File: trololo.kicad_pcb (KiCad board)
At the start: 4 copper layers, 136 x 54.8 mm, 101 parts, among them J1 USB_OTG, J10 Conn_02x12_Odd_Even, J11 Conn_02x02_Odd_Even, J13 PROTO1, J18 PROTO1, J2 USB_OTG, J3 Wuerth_7499010121A, J4 Micro_SD_Card, J5 Screw_Terminal_01x06, J6 Conn_02x12_Odd_Even, J7 USB_OTG, J8 Screw_Terminal_01x02, J9 Conn_02x12_Odd_Even, SW1 RESET, SW2 RESET, U1 STM32H743VITx, U10 USBLC6-2SC6, U11 SN6505, U2 KSZ8081RNA, U3 ISO1050DUB, U4 ISO3082DW, U5 W25Q32JVZP, U6 APE1707H-33-HF, U7 USBLC6-2SC6, U8 STM32F042G6Ux, U9 USBLC6-2SC6, Y1 8MHz, Y2 32.768KHz, Y3 25MHz

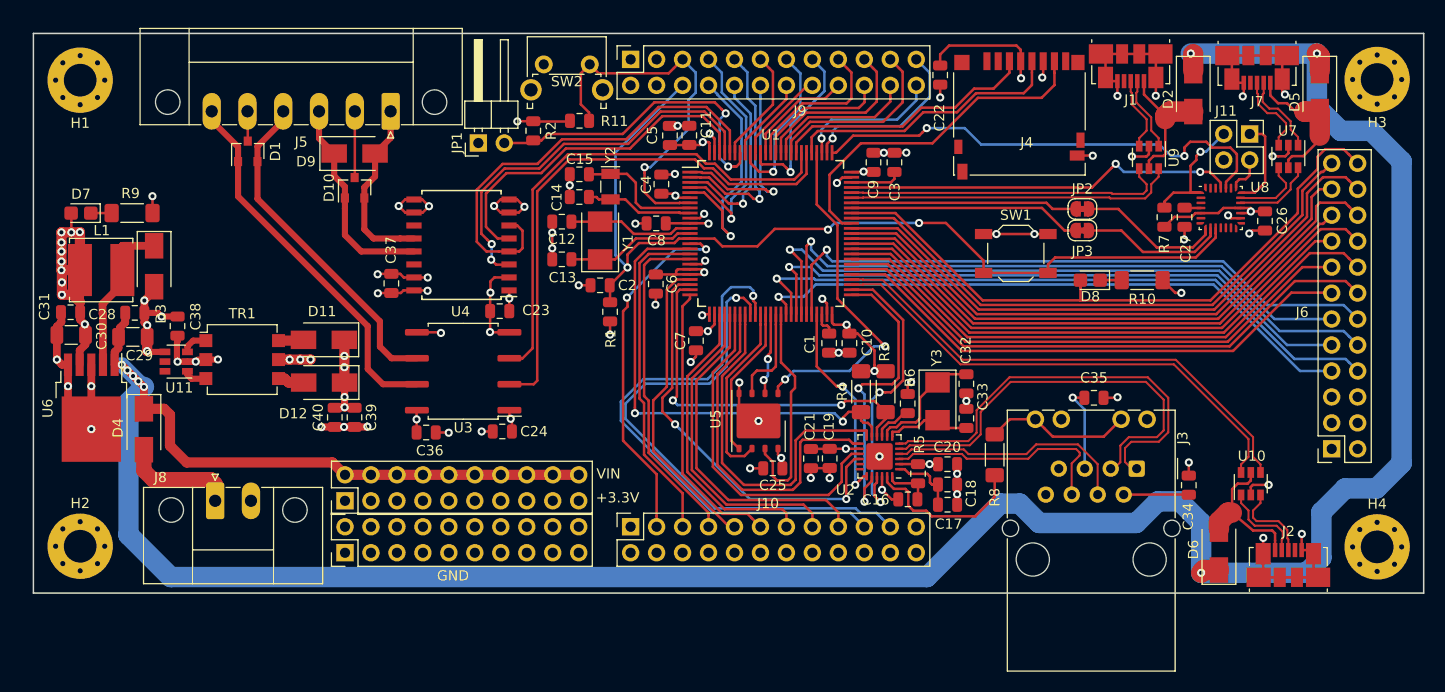
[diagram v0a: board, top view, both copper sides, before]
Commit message: Unknown changes
Signed-off-by: Martin Ribelotta <martinribelotta@gmail.com>
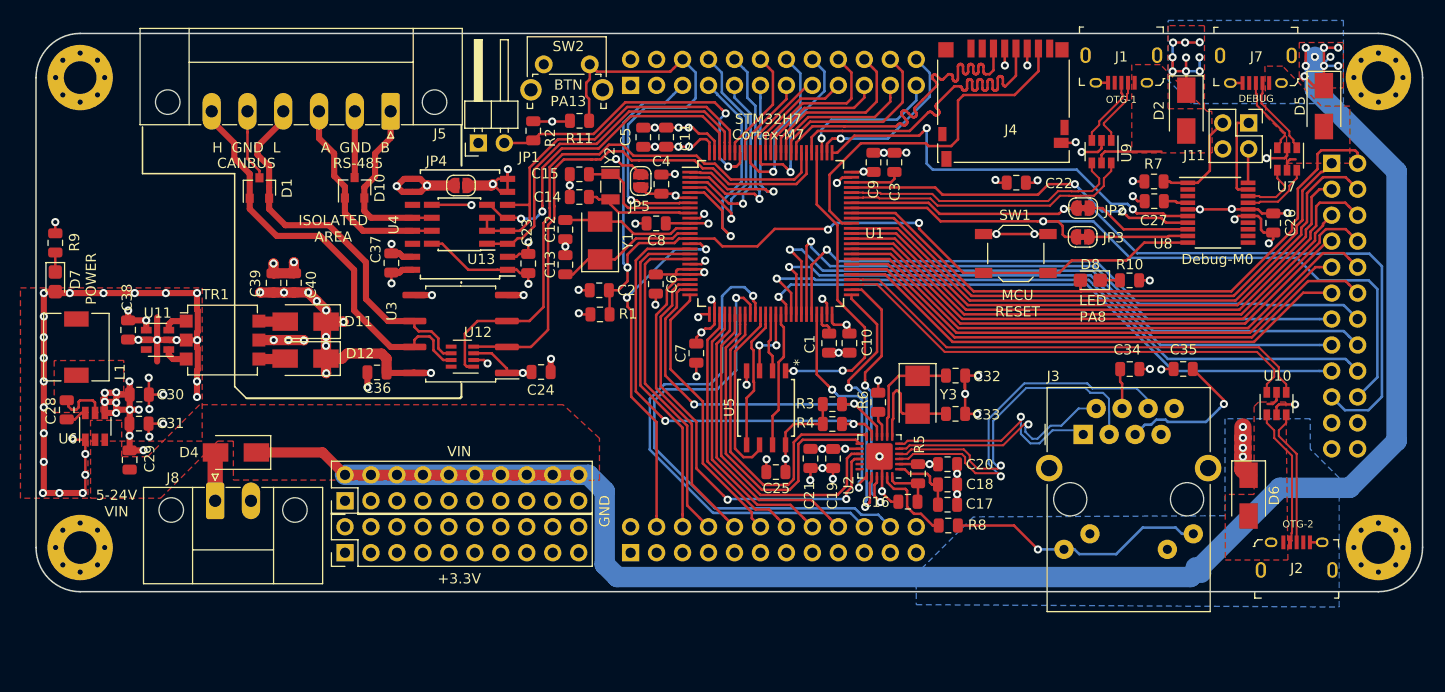
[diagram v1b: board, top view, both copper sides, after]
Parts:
- removed D3: D_Schottky_Small_ALT, Diode_SMD:D_SMA
- removed D9: D_TVS, Diode_SMD:D_SMA
- added JP4: Jumper_2_Bridged, Jumper:SolderJumper-2_P1.3mm_Open_RoundedPad1.0x1.5mm, F.Cu at (100.2, 42.8)
- added JP5: Jumper_2_Bridged, Jumper:SolderJumper-2_P1.3mm_Open_RoundedPad1.0x1.5mm, F.Cu at (117.8, 42.4)
- added U12: TCAN332, Package_TO_SOT_SMD:SOT-23-8, F.Cu at (100.4, 59.6)
- added U13: ISL83483, Package_SO:SOIC-8_3.9x4.9mm_P1.27mm, F.Cu at (100.1, 46.6)
- C29: value 470u -> 10u; footprint Capacitor_SMD:C_1206_3216Metric -> Capacitor_SMD:C_0805_2012Metric
- C30: value 470u -> 2.2u; footprint Capacitor_SMD:C_1206_3216Metric -> Capacitor_SMD:C_0805_2012Metric
- C31: value 0.1u -> 2.2u
- J1, J2, J7: value USB_OTG -> 10118194-0001LF; footprint Connector_USB:USB_Micro-B_Molex_47346-0001 -> footprints:USB_Micro_B_Female_10118194-0001LF
- J10, J6, J9: moved to B.Cu
- J3: value Wuerth_7499010121A -> RJ45_Amphenol_RJMG1BD3B8K1ANR; footprint Connector_RJ:RJ45_Wuerth_7499010121A_Horizontal -> Connector_RJ:RJ45_Amphenol_RJMG1BD3B8K1ANR
- L1: value L_Small -> 68uH; footprint Inductor_SMD:L_Bourns_SRN6045TA -> Inductor_SMD:L_6.3x6.3_H3
- R10, R3, R4, R8, R9: footprint Resistor_SMD:R_1806_4516Metric -> Resistor_SMD:R_0805_2012Metric
- SW2: value RESET -> PC13
- U5: value W25Q32JVZP -> S25FL127SABMFI101; footprint Package_SON:WSON-8-1EP_6x5mm_P1.27mm_EP3.4x4.3mm -> footprints:S25FL127SABMFI101
- U6: value APE1707H-33-HF -> AP63203; footprint Package_TO_SOT_SMD:TO-252-5_TabPin3 -> Package_TO_SOT_SMD:TSOT-23-6
- U8: value STM32F042G6Ux -> STM32F042F6Px; footprint Package_DFN_QFN:QFN-28_4x4mm_P0.5mm -> Package_SO:TSSOP-20_4.4x6.5mm_P0.65mm
- moved J6 27.9 mm to (185.4, 40.6)
- moved C39 15.3 mm to (81.9, 52.3), turned to 90 degrees
- moved C40 13.8 mm to (83.9, 52.3), turned to 90 degrees
- moved C22 12.9 mm to (154.6, 42.5), turned to 0 degrees
- moved C31 12.8 mm to (68.7, 66.1)
- moved C34 12.7 mm to (165.7, 60.8), turned to 180 degrees
- moved C29 12.0 mm to (67.8, 69.7), turned to 90 degrees
- moved C28 11.6 mm to (61.7, 64.8), turned to 90 degrees
- moved D4 9.29 mm to (78.2, 68.9), turned to 180 degrees
- moved C35 9.17 mm to (170.9, 60.8), turned to 0 degrees
- moved C30 8.86 mm to (68.8, 63.3)
- moved R8 8.27 mm to (147.9, 76.1), turned to 180 degrees
- moved U10 8.23 mm to (180.0, 64.2)
- moved R9 8.06 mm to (60.6, 48.4), turned to 270 degrees
- moved L1 7.92 mm to (62.6, 58.6), turned to 90 degrees
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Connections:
- C28 pad 1: VDC -> Net-(C28-Pad1)
- C28 pad 2: GND -> Net-(C28-Pad2)
- C4 pad 1: +3V3 -> +BATT
- J10 pad 10: GND -> /PA0
- J10 pad 11: /PA3 -> GND
- J10 pad 12: GND -> /PA3
- J10 pad 13: /PA4 -> GND
- J10 pad 14: GND -> /PA4
- J10 pad 15: /PA5 -> GND
- J10 pad 16: GND -> /PA5
- J10 pad 17: /PA6 -> GND
- J10 pad 18: GND -> /PA6
- J10 pad 19: /PB1 -> GND
- J10 pad 20: GND -> /PB1
- J10 pad 21: /PB0 -> GND
- J10 pad 22: GND -> /PB0
- J10 pad 3: /PC0 -> GND
- J10 pad 4: GND -> /PC0
- J10 pad 5: /PC2 -> GND
- J10 pad 6: GND -> /PC2
- J10 pad 7: /PC3 -> GND
- J10 pad 8: GND -> /PC3
- J10 pad 9: /PA0 -> GND
- J13 pad 1: GND -> +3V3
- J13 pad 11: GND -> +3V3
- J13 pad 13: GND -> +3V3
- J13 pad 15: GND -> +3V3
- J13 pad 17: GND -> +3V3
- J13 pad 19: GND -> +3V3
- J13 pad 3: GND -> +3V3
- J13 pad 5: GND -> +3V3
- J13 pad 7: GND -> +3V3
- J13 pad 9: GND -> +3V3
- J18 pad 1: +3V3 -> GND
- J18 pad 11: +3V3 -> GND
- J18 pad 13: +3V3 -> GND
- J18 pad 15: +3V3 -> GND
- J18 pad 17: +3V3 -> GND
- J18 pad 19: +3V3 -> GND
- J18 pad 3: +3V3 -> GND
- J18 pad 5: +3V3 -> GND
- J18 pad 7: +3V3 -> GND
- J18 pad 9: +3V3 -> GND
- J6 pad 1: GND -> /PC9
- J6 pad 10: /PE14 -> /PD11
- J6 pad 11: /PE15 -> /PD8
- J6 pad 12: /PB10 -> /PD9
- J6 pad 13: /PD8 -> /PE15
- J6 pad 14: /PD9 -> /PB10
- J6 pad 15: /PD10 -> /PE13
- J6 pad 16: /PD11 -> /PE14
- J6 pad 17: /PD12 -> /PE11
- J6 pad 18: /PD13 -> /PE12
- J6 pad 19: /PD14 -> /U1_RX
- J6 pad 2: +3V3 -> /PA8
- J6 pad 20: /PD15 -> /U1_TX
- J6 pad 21: /PC6 -> GND
- J6 pad 22: /PC7 -> +3V3
- J6 pad 23: /PC9 -> GND
- J6 pad 24: /PA8 -> +3V3
- J6 pad 3: GND -> /PC6
- J6 pad 4: +3V3 -> /PC7
- J6 pad 5: GND -> /PD14
- J6 pad 6: +3V3 -> /PD15
- J6 pad 7: /PE11 -> /PD12
- J6 pad 8: /PE12 -> /PD13
- J6 pad 9: /PE13 -> /PD10
- J9 pad 1: +3V3 -> GND
- J9 pad 10: /PE4 -> /PE3
- J9 pad 11: /PB8 -> /PE2
- J9 pad 12: /PE2 -> /PB8
- J9 pad 13: /PB6 -> /PB7
- J9 pad 14: /PB7 -> /PB6
- J9 pad 15: /PB4 -> /PB5
- J9 pad 16: /PB5 -> /PB4
- J9 pad 17: /PD7 -> /PB3
- J9 pad 18: /PB3 -> /PD7
- J9 pad 19: /PD5 -> /PD6
- J9 pad 2: GND -> +3V3
- J9 pad 20: /PD6 -> /PD5
- J9 pad 21: /PD3 -> /PD4
- J9 pad 22: /PD4 -> /PD3
- J9 pad 23: /PA15 -> /PC10
- J9 pad 24: /PC10 -> /PA15
- J9 pad 3: +3V3 -> +BATT
- J9 pad 4: GND -> +3V3
- J9 pad 5: /PC13 -> /~RESET
- J9 pad 6: /~RESET -> /PC13
- J9 pad 7: /PE5 -> /PE6
- J9 pad 8: /PE6 -> /PE5
- J9 pad 9: /PE3 -> /PE4
- L1 pad 1: Net-(D3-Pad1) -> Net-(C28-Pad2)
- R8 pad 1: Net-(J3-Pad10) -> Net-(J3-PadL1)
- U1 pad 6: +3V3 -> +BATT
- U11 pad 5: Net-(U11-Pad5) -> +3V3
- U6 pad 1: VDC -> +3V3
- U6 pad 2: Net-(D3-Pad1) -> VDC
- U6 pad 3: GND -> VDC
- U6 pad 4: +3V3 -> GND
- U6 pad 5: GND -> Net-(C28-Pad2)
- U8 pad 15: Net-(U8-Pad15) -> GND
- U8 pad 16: GND -> +3V3
- U8 pad 17: +3V3 -> /USB_SER_D-
- U8 pad 18: +3V3 -> /USB_SER_D+
- U8 pad 19: /USB_SER_D- -> /SWDIO_B
- U8 pad 20: /USB_SER_D+ -> /SWCLK_B
- U8 pad 6: Net-(U8-Pad6) -> /SWCLK
- U8 pad 7: Net-(U8-Pad7) -> /SWDIO
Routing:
- net VDC: track 283.1 -> 224.5 mm, vias 8 -> 22
- net /U1_RX: track 22.2 -> 74.9 mm, vias 0 -> 1
- net +3V3: track 116.1 -> 164.3 mm, vias 30 -> 54
- net /U1_TX: track 22.8 -> 70.4 mm, vias 0 -> 1
- net GND: track 172.8 -> 133.9 mm, vias 63 -> 65
- net Net-(J3-PadL1): track 0.00 -> 25.5 mm, vias 0 -> 1
- net /TD+: track 42.2 -> 22.1 mm, vias 0 -> 1
- net +BATT: track 0.00 -> 18.8 mm, vias 0 -> 1
- net /TD-: track 41.3 -> 22.9 mm, vias 0 -> 1
- net /VBUS2: track 18.0 -> 1.73 mm
- net Net-(D3-Pad1): track 15.6 -> 0.00 mm
- net +5P: track 15.8 -> 30.5 mm, vias 7 -> 11
- net Net-(J3-Pad10): track 14.4 -> 0.00 mm
- net /RD-: track 23.0 -> 36.0 mm, vias 0 -> 1
- net /VBUS3: track 14.2 -> 1.80 mm
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- added copper zone on F.Cu, net +3V3
- added copper zone on F.Cu, net /VBUS1
- added copper zone on F.Cu, net /VBUS2
- added copper zone on F.Cu, net /VBUS3
- added copper zone on F.Cu, net Net-(C28-Pad2)
- added copper zone on B.Cu, net VDC
- added copper zone on F.Cu, net VDC
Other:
- board size 136 x 54.8 mm -> 135.6 x 54.6 mm
- board text added: "5-24V VIN"
- board text added: "A GND B"
- board text added: "BTN PA13"
- board text added: "CANBUS"
- board text added: "Cortex-M7"
- board text added: "DEBUG"
- board text added: "Debug-M0"
- board text added: "H GND L"
- board text added: "ISOLATED AREA"
- board text added: "LED PA8"
- board text added: "MCU RESET"
- board text added: "OTG-1"
- board text added: "OTG-2"
- board text added: "POWER"
- board text added: "RS-485"
- board text added: "STM32H7"
